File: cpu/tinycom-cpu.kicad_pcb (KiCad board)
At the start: 4 copper layers, 39.9 x 41.4 mm, 10 parts, among them P1 CONN_02X08, P2 CONN_02X08, U1 OLIMEX_IC_A13, U2 H5TQG63BFR/FBGA96, Y1 Crystal

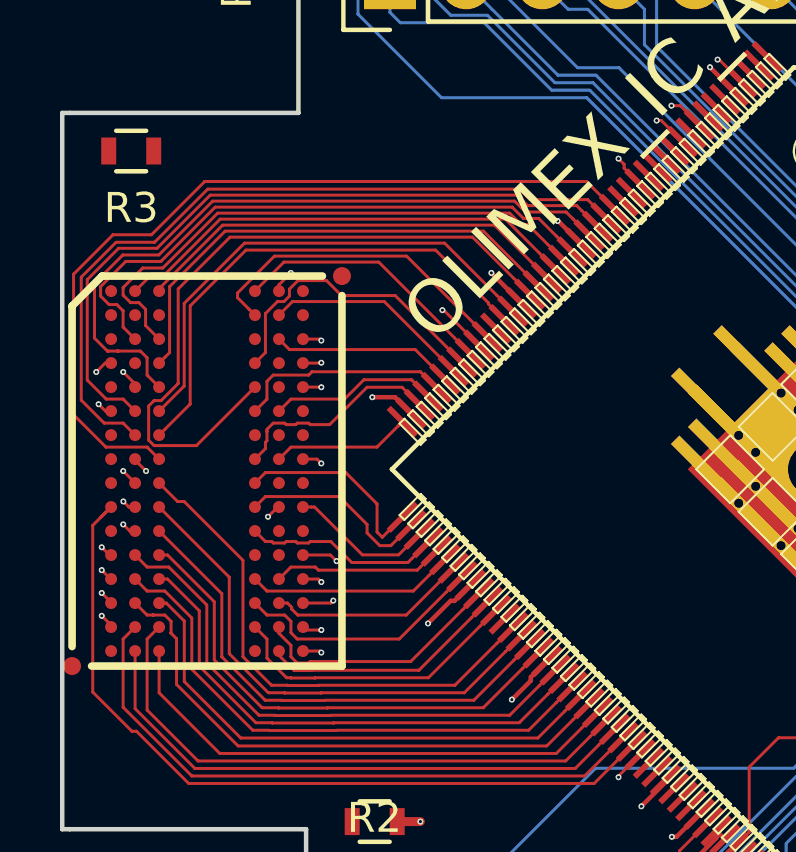
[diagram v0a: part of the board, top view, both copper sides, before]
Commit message: full ddr route
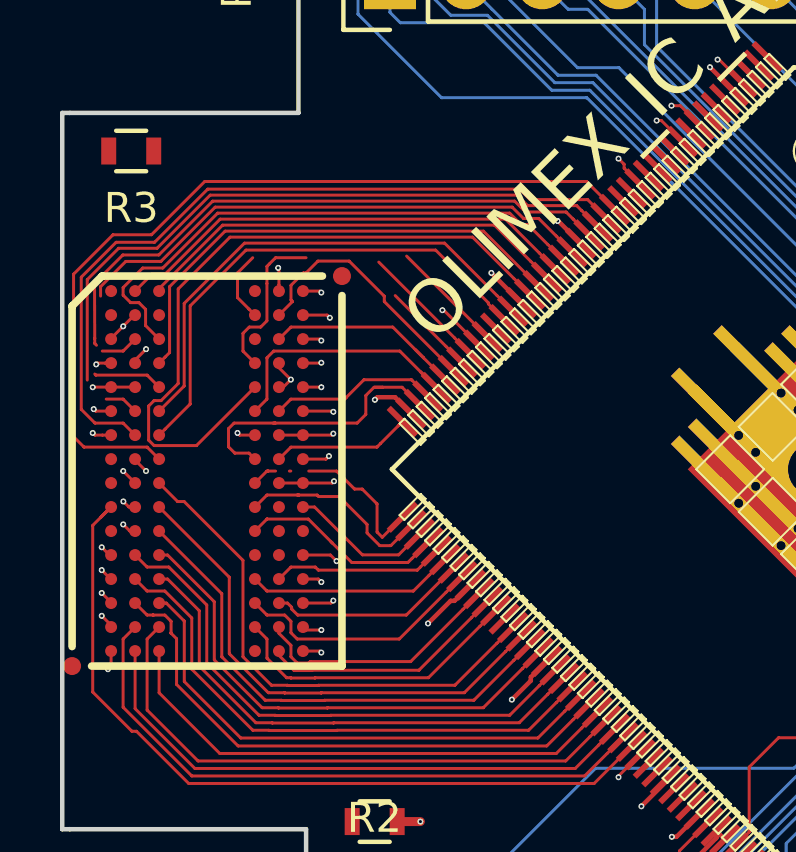
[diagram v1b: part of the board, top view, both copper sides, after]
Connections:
- U2 pad J9: Net-(U2-PadJ9) -> GND
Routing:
- net GND: track 7.14 -> 17.0 mm, vias 10 -> 18
- net DDR_DQS1_N: track 10.9 -> 6.17 mm
- net DDR_D12: track 8.85 -> 4.32 mm
- net DDR_D7: track 7.14 -> 9.54 mm
- net DDR_D1: track 7.16 -> 8.94 mm
- net DDR_D14: track 6.96 -> 8.57 mm
- net DDR_D8: track 10.1 -> 8.51 mm
- net DDR_CK_P: track 6.78 -> 5.72 mm
- net DDR_D2: track 24.0 -> 23.1 mm
- net DDR_D11: track 19.8 -> 19.0 mm
- net DDR_D10: track 6.08 -> 6.81 mm
- net DDR_D0: track 23.2 -> 22.5 mm
- net VCC_15: track 62.7 -> 63.0 mm, vias 19 -> 21
